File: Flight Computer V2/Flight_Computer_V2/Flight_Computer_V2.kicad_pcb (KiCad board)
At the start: 4 copper layers, 90.2 x 95.9 mm, 151 parts, among them IC1 MB85RC256VPF-G-JNERE2, IC2 MB85RC256VPF-G-JNERE2, IC3 MB85RC256VPF-G-JNERE2, IC4 MB85RC256VPF-G-JNERE2, IC5 BMI088, IC6 MMC5603NJ, IC7 MAX31855KASA+T, IC8 MAX31855KASA+T, IC9 MAX31855KASA+T, J2 Conn_02x26_Odd_Even, J4 Conn_02x26_Odd_Even, U1 STM32F405RGTx, U3 MCP2562-E-SN, U44 BMP280

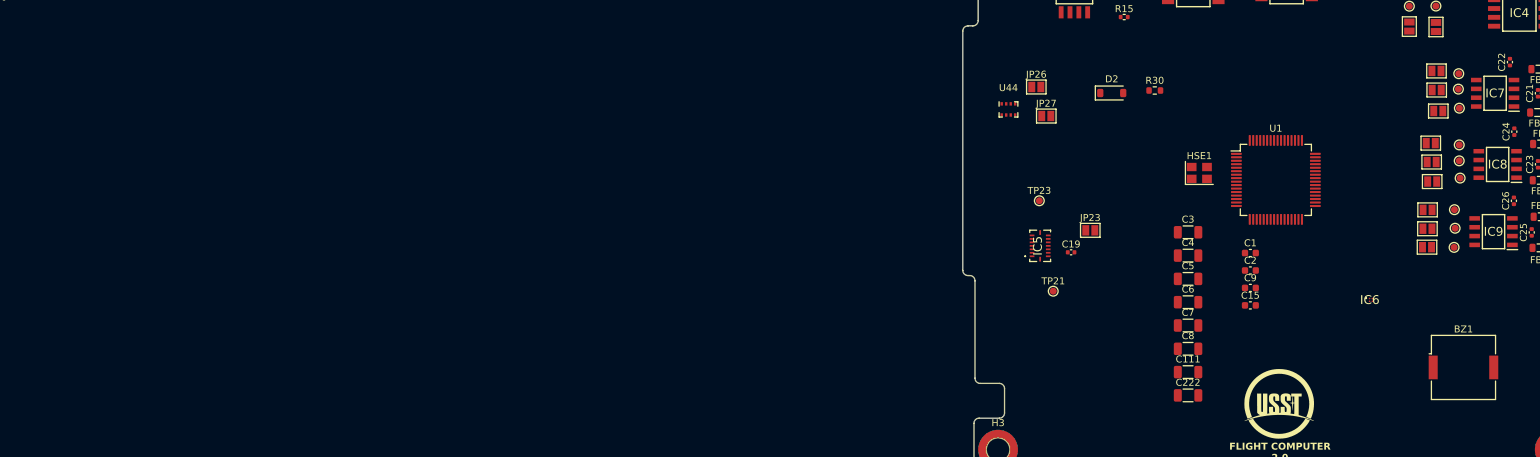
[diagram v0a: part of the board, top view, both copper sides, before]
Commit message: updated v2 flight computer
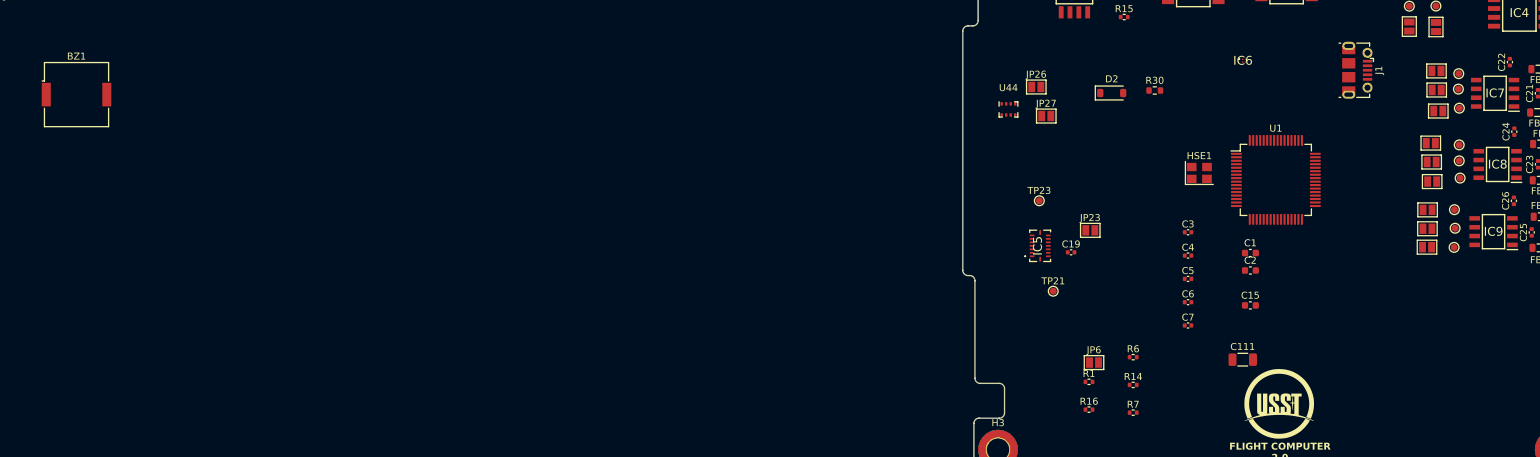
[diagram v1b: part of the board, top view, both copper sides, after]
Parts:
- removed C222, C8: 100u, Capacitor_SMD:C_1206_3216Metric
- removed C9: 10u, Capacitor_SMD:C_0603_1608Metric
- added J1: USB_B_Micro, Connector_USB:USB_Micro-B_Molex-105017-0001, F.Cu at (158.7, 75.2)
- added JP6: ~, Jumper:SolderJumper-2_P1.3mm_Open_Pad1.0x1.5mm, F.Cu at (120.9, 117.3)
- added R1: 10k, Resistor_SMD:R_0402_1005Metric, F.Cu at (120.1, 120.0)
- added R14: 10k, Resistor_SMD:R_0402_1005Metric, F.Cu at (126.5, 120.5)
- added R16: 10k, Resistor_SMD:R_0402_1005Metric, F.Cu at (120.1, 124.0)
- added R6: 10k, Resistor_SMD:R_0402_1005Metric, F.Cu at (126.5, 116.5)
- added R7: 10k, Resistor_SMD:R_0402_1005Metric, F.Cu at (126.5, 124.5)
- C111: value 100u -> 4u7
- C3, C4, C5, C6, C7: value 100u -> 100n; footprint Capacitor_SMD:C_1206_3216Metric -> Capacitor_SMD:C_0402_1005Metric
- moved BZ1 203.2 mm to (-25.4, 78.7)
- moved IC6 38.9 mm to (142.4, 73.9)
- moved C111 8.06 mm to (142.2, 116.8)
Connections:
- C111 pad 2: GND -> Net-(C111-Pad2)
- C3 pad 2: GND -> Net-(C111-Pad2)
- C4 pad 2: GND -> Net-(C111-Pad2)
- C5 pad 2: GND -> Net-(C111-Pad2)
- C6 pad 2: GND -> Net-(C111-Pad2)
- C7 pad 2: GND -> Net-(C111-Pad2)
